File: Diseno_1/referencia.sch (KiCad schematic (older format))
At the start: 12 parts, among them J1 Conn_01x06, J2 USB_B_Micro, SW1 SW_Push, U5 XC7Z010-BUENO, U8 CP2102N-A01-GQFN28

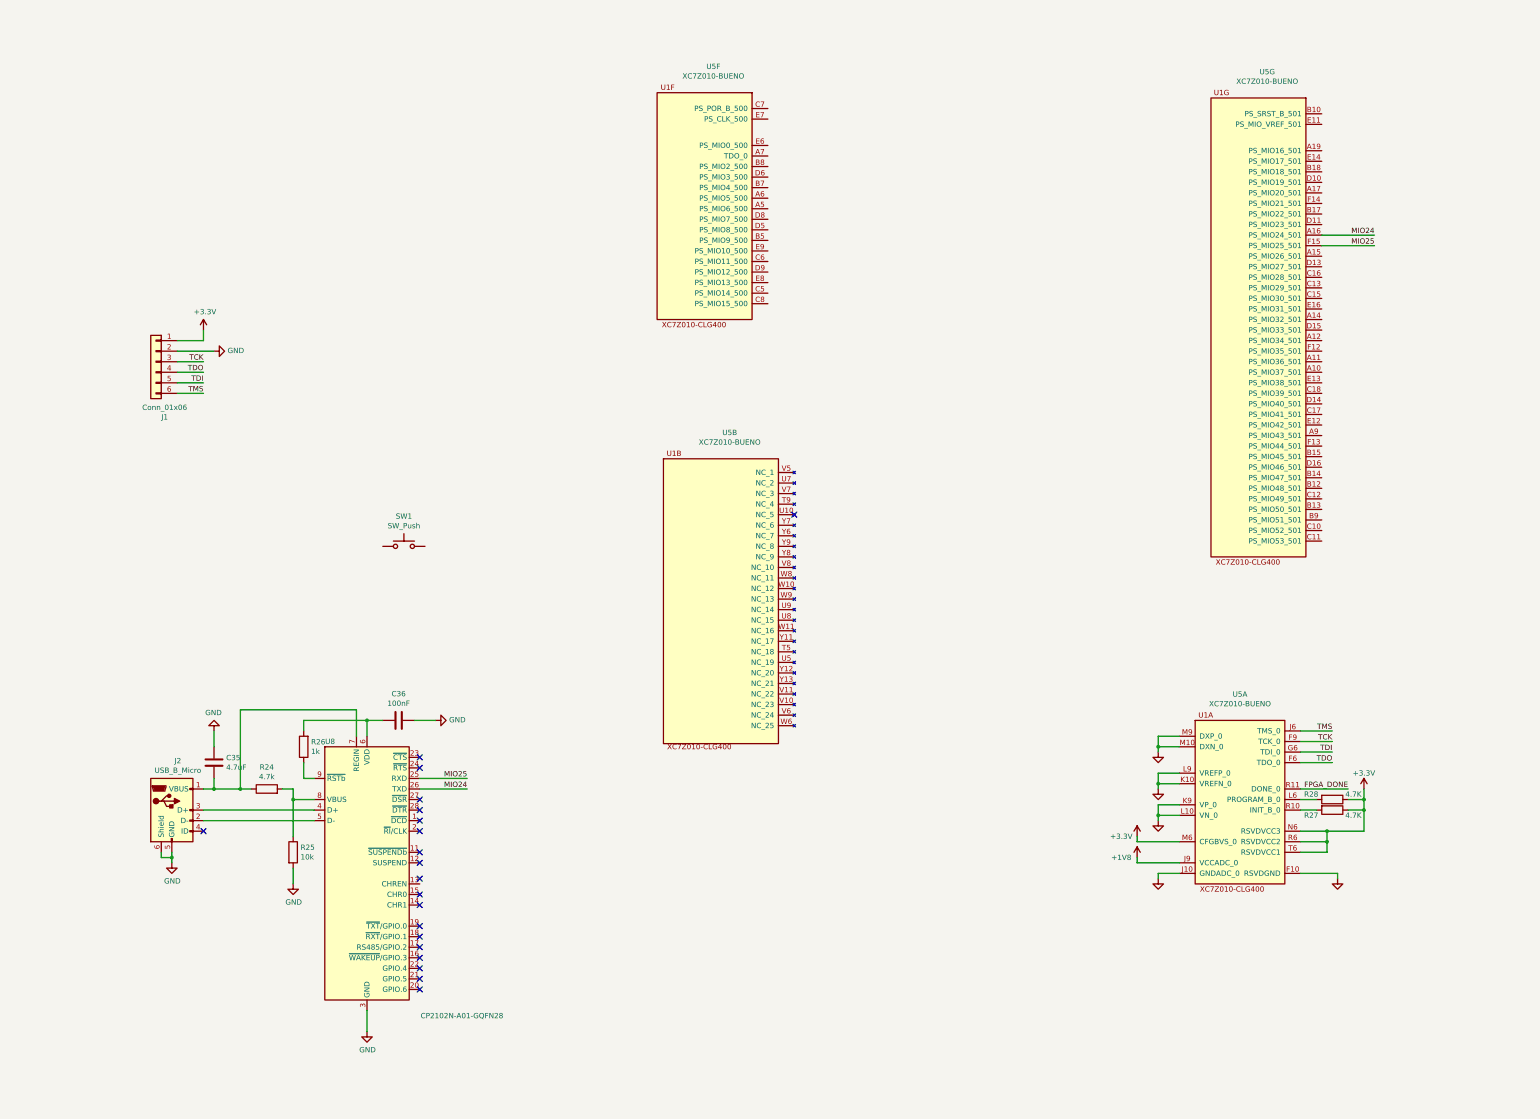
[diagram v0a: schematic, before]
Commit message: muchas cosas
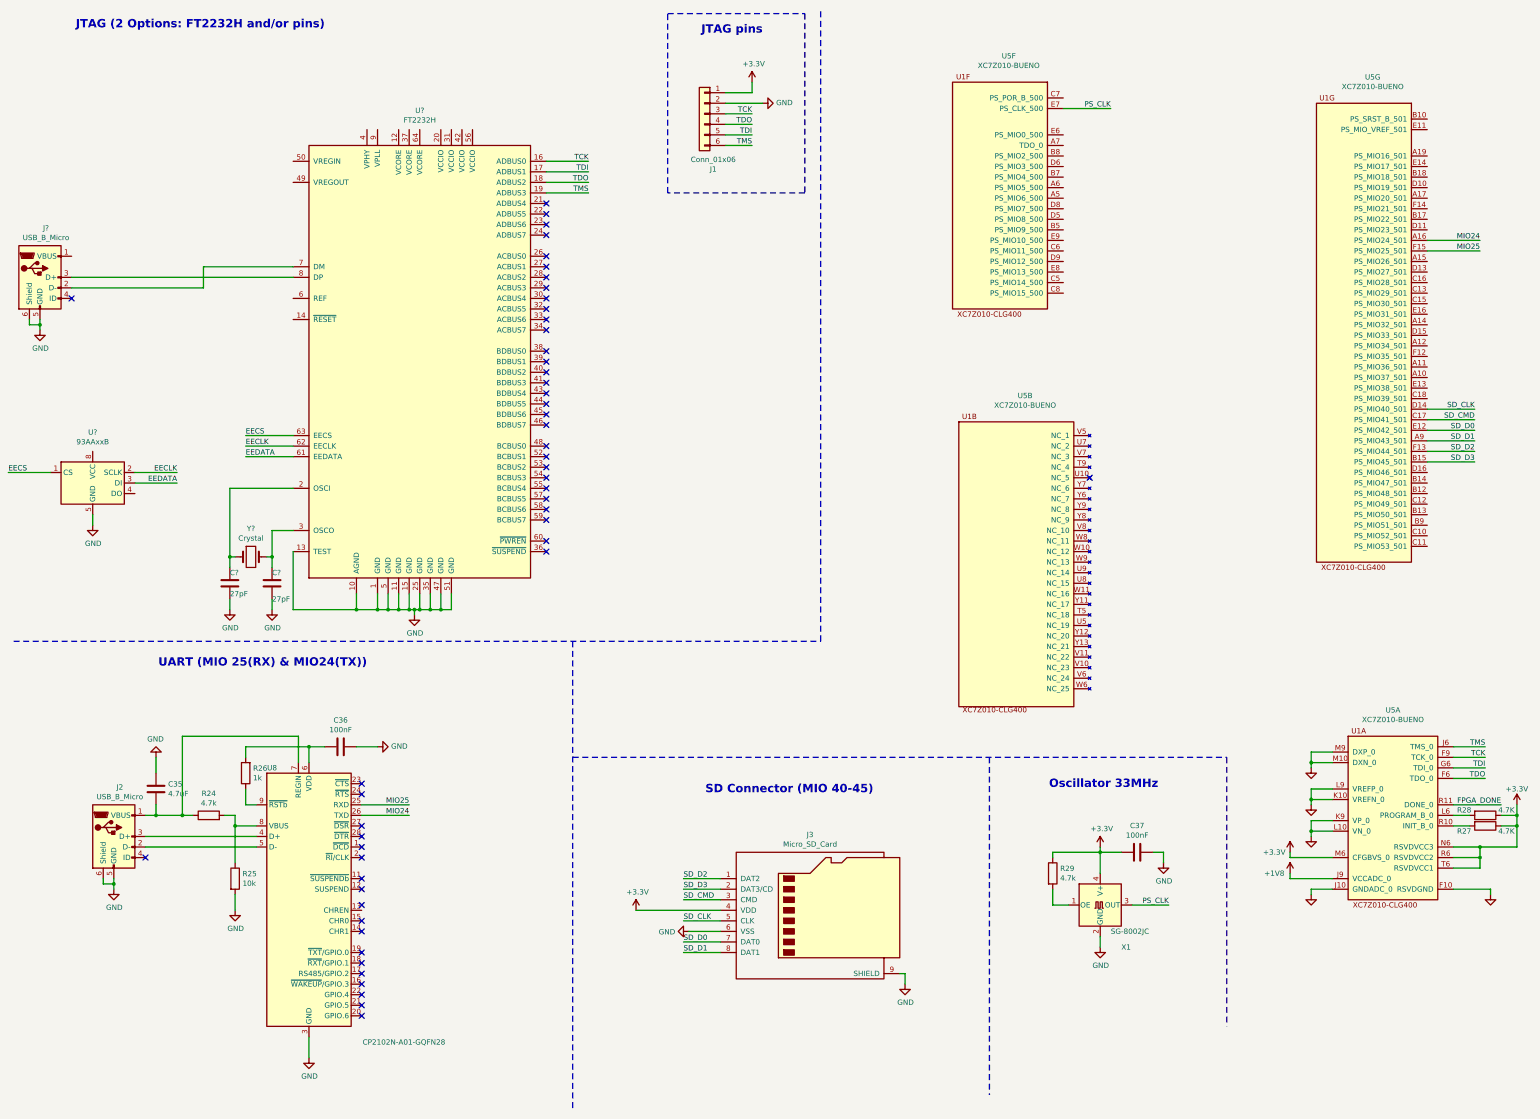
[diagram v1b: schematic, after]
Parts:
- removed SW1: SW_Push, Button_Switch_SMD:SW_SPST_CK_RS282G05A3, symbol Switch:SW_Push
- added C37: 100nF, Capacitor_SMD:C_0805_2012Metric, symbol Device:C
- added C? (x2): 27pF, Capacitor_SMD:C_0805_2012Metric, symbol Device:C
- added J3: Micro_SD_Card, Connector_Card:microSD_HC_Wuerth_693072010801, symbol Connector:Micro_SD_Card
- added J?: USB_B_Micro, Connector_USB:USB_Mini-B_Lumberg_2486_01_Horizontal, symbol Connector:USB_B_Micro
- added R29: 4.7k, Resistor_SMD:R_0805_2012Metric, symbol Device:R
- added U?: FT2232H, Package_QFP:LQFP-64-1EP_10x10mm_P0.5mm_EP6.5x6.5mm, symbol Interface_USB:FT2232H
- added U?: 93AAxxB, symbol Memory_EEPROM:93AAxxB
- added X1: SG-8002JC, Oscillator:Oscillator_SMD_SeikoEpson_SG8002JC-4Pin_10.5x5.0mm, symbol Oscillator:SG-8002JC
- added Y?: Crystal, Crystal:Crystal_SMD_0603-2Pin_6.0x3.5mm, symbol Device:Crystal
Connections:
- net +3V3: now also C37.2, J3.4 (VDD), R29.1, X1.4 (V+)
- net GND: now also C37.1, C?.2, C?.2, J3.6 (VSS), J3.9 (SHIELD), J?.5 (GND), J?.6 (Shield), U?.1 (GND), U?.10 (AGND), U?.11 (GND), U?.13 (TEST), U?.15 (GND), U?.25 (GND), U?.35 (GND), U?.47 (GND), U?.5 (GND), U?.5 (GND), U?.51 (GND), X1.2 (GND)
- net TCK: now also U?.16 (ADBUS0)
- net TDI: now also U?.17 (ADBUS1)
- net TDO: now also U?.18 (ADBUS2)
- net TMS: now also U?.19 (ADBUS3)
- net PS_CLK: now reaches U5.E7 (PS_CLK_500)
- net PS_CLK: now also X1.3 (OUT)
- net SD_D1: now reaches U5.A9 (PS_MIO43_501)
- net SD_D1: now also J3.8 (DAT1)
- net SD_D3: now reaches U5.B15 (PS_MIO45_501)
- net SD_D3: now also J3.2 (DAT3/CD)
- net SD_CMD: now reaches U5.C17 (PS_MIO41_501)
- net SD_CMD: now also J3.3 (CMD)
- net SD_CLK: now reaches U5.D14 (PS_MIO40_501)
- net SD_CLK: now also J3.5 (CLK)
- net SD_D0: now reaches U5.E12 (PS_MIO42_501)
- net SD_D0: now also J3.7 (DAT0)
- net SD_D2: now reaches U5.F13 (PS_MIO44_501)
- net SD_D2: now also J3.1 (DAT2)
- new net: R29.2, X1.1 (OE)
- new net: C?.1, U?.2 (OSCI), Y?.1
- new net: C?.1, U?.3 (OSCO), Y?.2
- new net: J?.2 (D-), U?.7 (DM)
- new net: J?.3 (D+), U?.8 (DP)
- new net EECLK: U?.2 (SCLK), U?.62 (EECLK)
- new net EECS: U?.1 (CS), U?.63 (EECS)
- new net EEDATA: U?.3 (DI), U?.61 (EEDATA)
- no-connect marks 20 -> 51
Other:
- note added: "JTAG (2 Options: FT2232H and/or pins)"
- note added: "JTAG pins"
- note added: "Oscillator 33MHz\n"
- note added: "SD Connector (MIO 40-45)\n"
- note added: "UART (MIO 25(RX) & MIO24(TX))"
- moved on the sheet: C35, C36, J1, J2, R24, R25, R26, R27, R28, U5A, U5B, U5F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
